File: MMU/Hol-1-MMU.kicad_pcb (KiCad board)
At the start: 2 copper layers, 106.7 x 76.2 mm, 28 parts, among them P1 DATA BUS, P2 ADDRESS PORT, P3 DATA PORT, P4 MMU CONTROL, P5 Power, SW1 HEX_SWITCH, SW2 HEX_SWITCH, SW3 HEX_SWITCH, SW4 HEX_SWITCH, SW5 DPDT, SW6 SW_PUSH, U1 74LS00, U2 74LS173, U3 74LS157, U4 74LS173, U5 74LS157, U6 74LS157, U7 74LS157, U8 74LS157

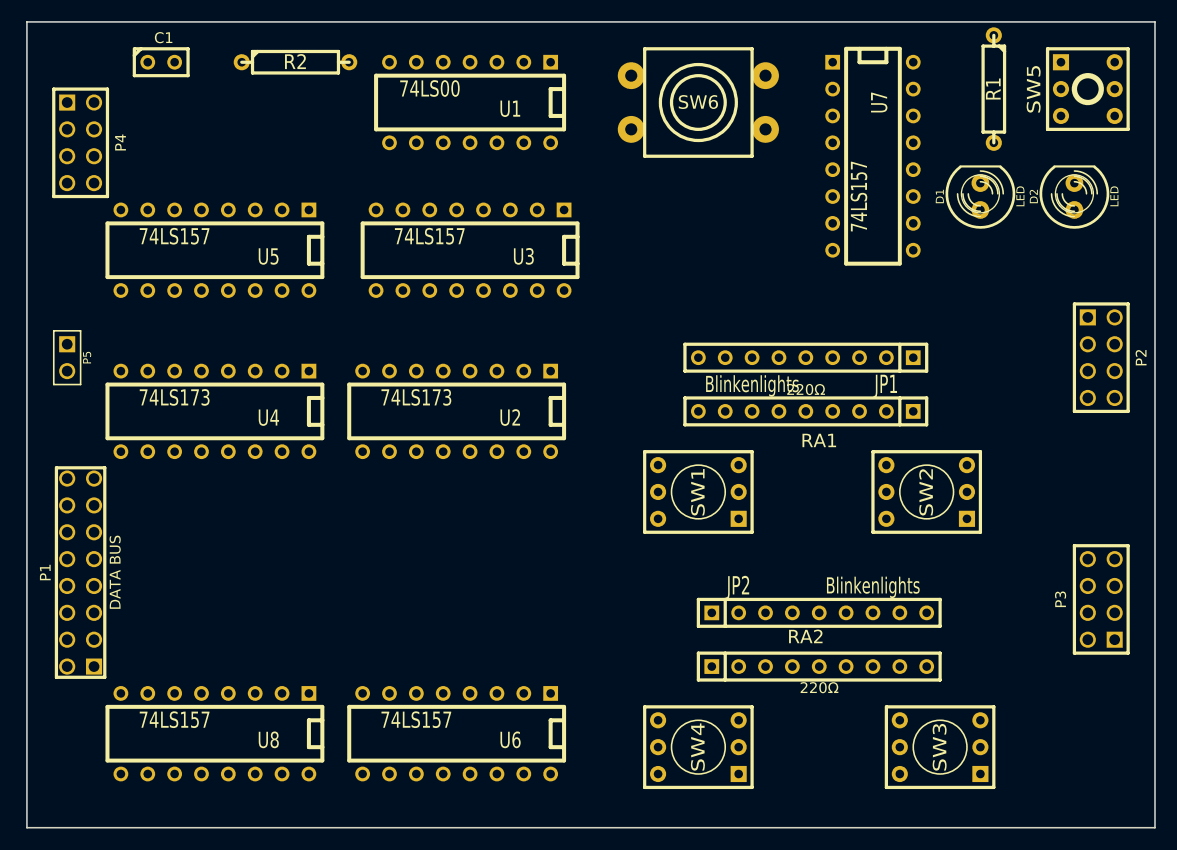
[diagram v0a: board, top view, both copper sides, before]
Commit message: v1.5.3 initial MMU board layout
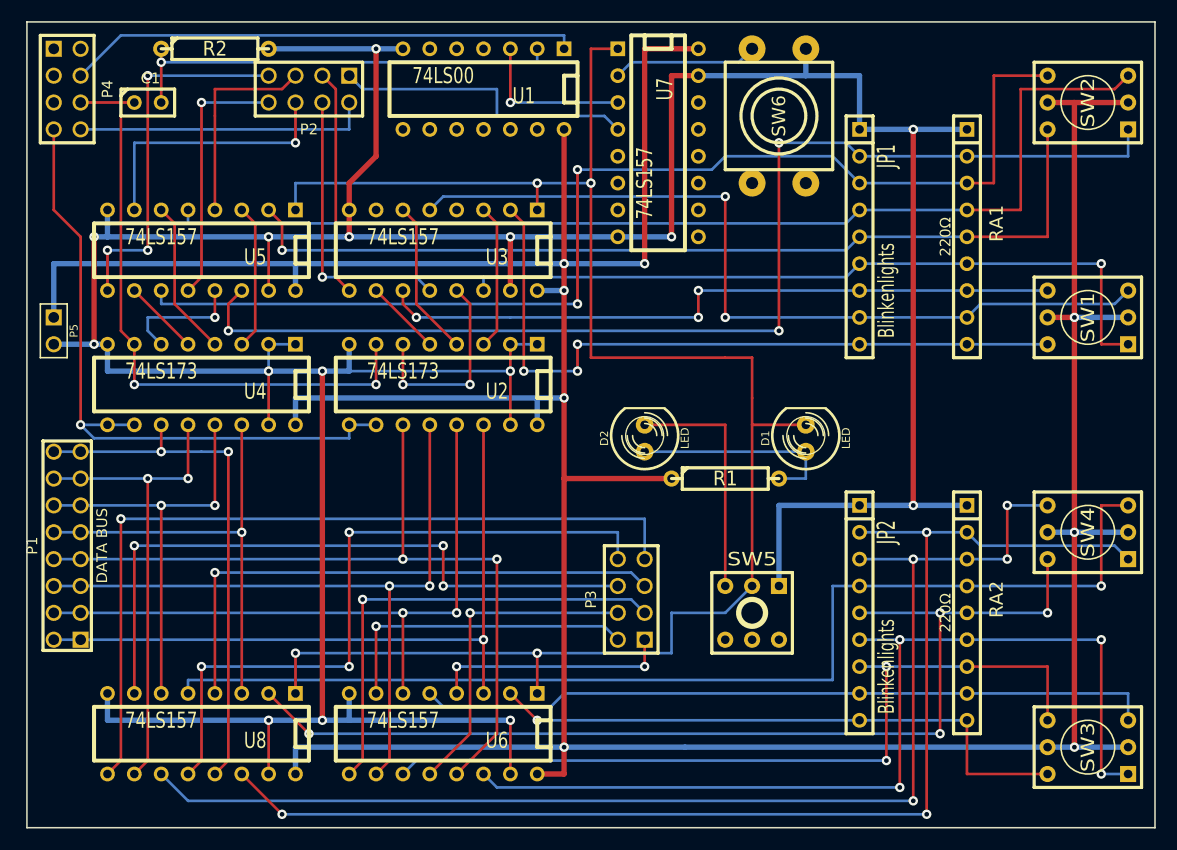
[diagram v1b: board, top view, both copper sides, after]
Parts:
- moved P2 79.1 mm to (130.8, 69.8), turned to 180 degrees
- moved SW5 58.8 mm to (172.7, 119.4), turned to 180 degrees
- moved D2 46.6 mm to (162.6, 102.9)
- moved R1 44.7 mm to (170.2, 106.7), turned to 0 degrees
- moved P3 44.5 mm to (161.3, 118.1)
- moved SW4 42.1 mm to (204.5, 111.8)
- moved SW1 40.4 mm to (204.5, 91.4)
- moved SW2 39.9 mm to (204.5, 71.1)
- moved D1 28.2 mm to (177.8, 102.9)
- moved RA1 22.5 mm to (193.0, 83.8), turned to 270 degrees
- moved U7 20.4 mm to (163.8, 74.9)
- moved RA2 14.9 mm to (193.0, 119.4), turned to 270 degrees
- moved SW3 14.0 mm to (204.5, 132.1)
- moved JP1 12.5 mm to (182.9, 83.8), turned to 270 degrees
- moved SW6 7.73 mm to (175.3, 72.4), turned to 270 degrees
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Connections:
- P4 pad 1: /RAM-INPUT -> (no net)
- P4 pad 2: /CLK -> (no net)
- P4 pad 4: (no net) -> /RAM-INPUT
- P4 pad 6: (no net) -> /CLK
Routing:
- net GND: track 0.00 -> 375.7 mm, vias 0 -> 15
- net +5V: track 0.00 -> 360.7 mm, vias 0 -> 8
- net /PROG: track 0.00 -> 162.3 mm, vias 0 -> 4
- net N-0000049: track 0.00 -> 119.5 mm, vias 0 -> 3
- net N-0000050: track 0.00 -> 117.9 mm, vias 0 -> 4
- net N-0000010: track 0.00 -> 110.3 mm, vias 0 -> 3
- net N-000006: track 0.00 -> 109.5 mm, vias 0 -> 2
- net N-0000056: track 0.00 -> 106.7 mm, vias 0 -> 1
- net N-000002: track 0.00 -> 102.7 mm
- net N-0000062: track 0.00 -> 99.4 mm, vias 0 -> 4
- net N-0000063: track 0.00 -> 92.0 mm, vias 0 -> 4
- net N-000003: track 0.00 -> 87.4 mm, vias 0 -> 1
- net N-000001: track 0.00 -> 79.0 mm, vias 0 -> 2
- net N-0000064: track 0.00 -> 78.0 mm, vias 0 -> 2
- net N-0000040: track 0.00 -> 78.0 mm, vias 0 -> 1
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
